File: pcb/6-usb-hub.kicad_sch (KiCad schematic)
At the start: 19 parts, among them J601 USB-C (HRO TYPE-C-31-M-12), U601 CH334P, Y601 12MHz ABM8-272-T3

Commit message: Phase 3: footprint audit fixes and project footprint library
- New project footprint library pcb/scsi-adapter.pretty, generated by
  pcb/_gen/footprints.py from datasheet land patterns: TI RPW0010A (U101/U201),
  Kangnex WJ500V (J101), TE AMPLIMITE .050 HD50 (J302), SHOU HAN TF PUSH
  microSD (J501), Abracon AOTA-B201610 polarized inductor (L401), SHOU HAN
  2-pos DIP (SW301). fp-lib-table added.
- J303 LA header: 2x17 box header C20920, pins 33/34 NC (34-way ribbon to a
  future 2x16 adapter board).
- J302 HD50: TE 5787082-5 squeeze-latch receptacle; shielded symbol, shell to
  GND via R343 0R. TE STEP model git-ignored (pcb/scsi-adapter.3dshapes/).
- D101/D204/D605: D_SMF -> D_SOD-123F (parts are SOD-123FL).
- L401 pins swapped so pad 1 = polarity dot = DVDD_1V1 (RP2350 Fig. 23).
- SW401/SW402: Hroparts K2-1102DP C110153 on SW_PUSH_6mm.
- NOTES, decisions, sources updated; J601 pad question closed; RP2350B
  minimal-design layout copy planned (open question 17).
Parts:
- D605: footprint Diode_SMD:D_SMF -> Diode_SMD:D_SOD-123F
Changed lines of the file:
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@@
 		(property "Reference" "D605" (at 147.32 237.49 270) (effects (font (size 1.27 1.27)) (justify right)))
 		(property "Value" "SMF6.0A" (at 147.32 240.03 270) (effects (font (size 1.27 1.27)) (justify right)))
-		(property "Footprint" "Diode_SMD:D_SMF" (at 144.78 238.76 0) (effects (font (size 1.27 1.27)) (hide yes)))
+		(property "Footprint" "Diode_SMD:D_SOD-123F" (at 144.78 238.76 0) (effects (font (size 1.27 1.27)) (hide yes)))
 		(property "Datasheet" "" (at 144.78 238.76 0) (effects (font (size 1.27 1.27)) (hide yes)))
 		(property "Description" "ESD on VBUS" (at 144.78 238.76 0) (effects (font (size 1.27 1.27)) (hide yes)))

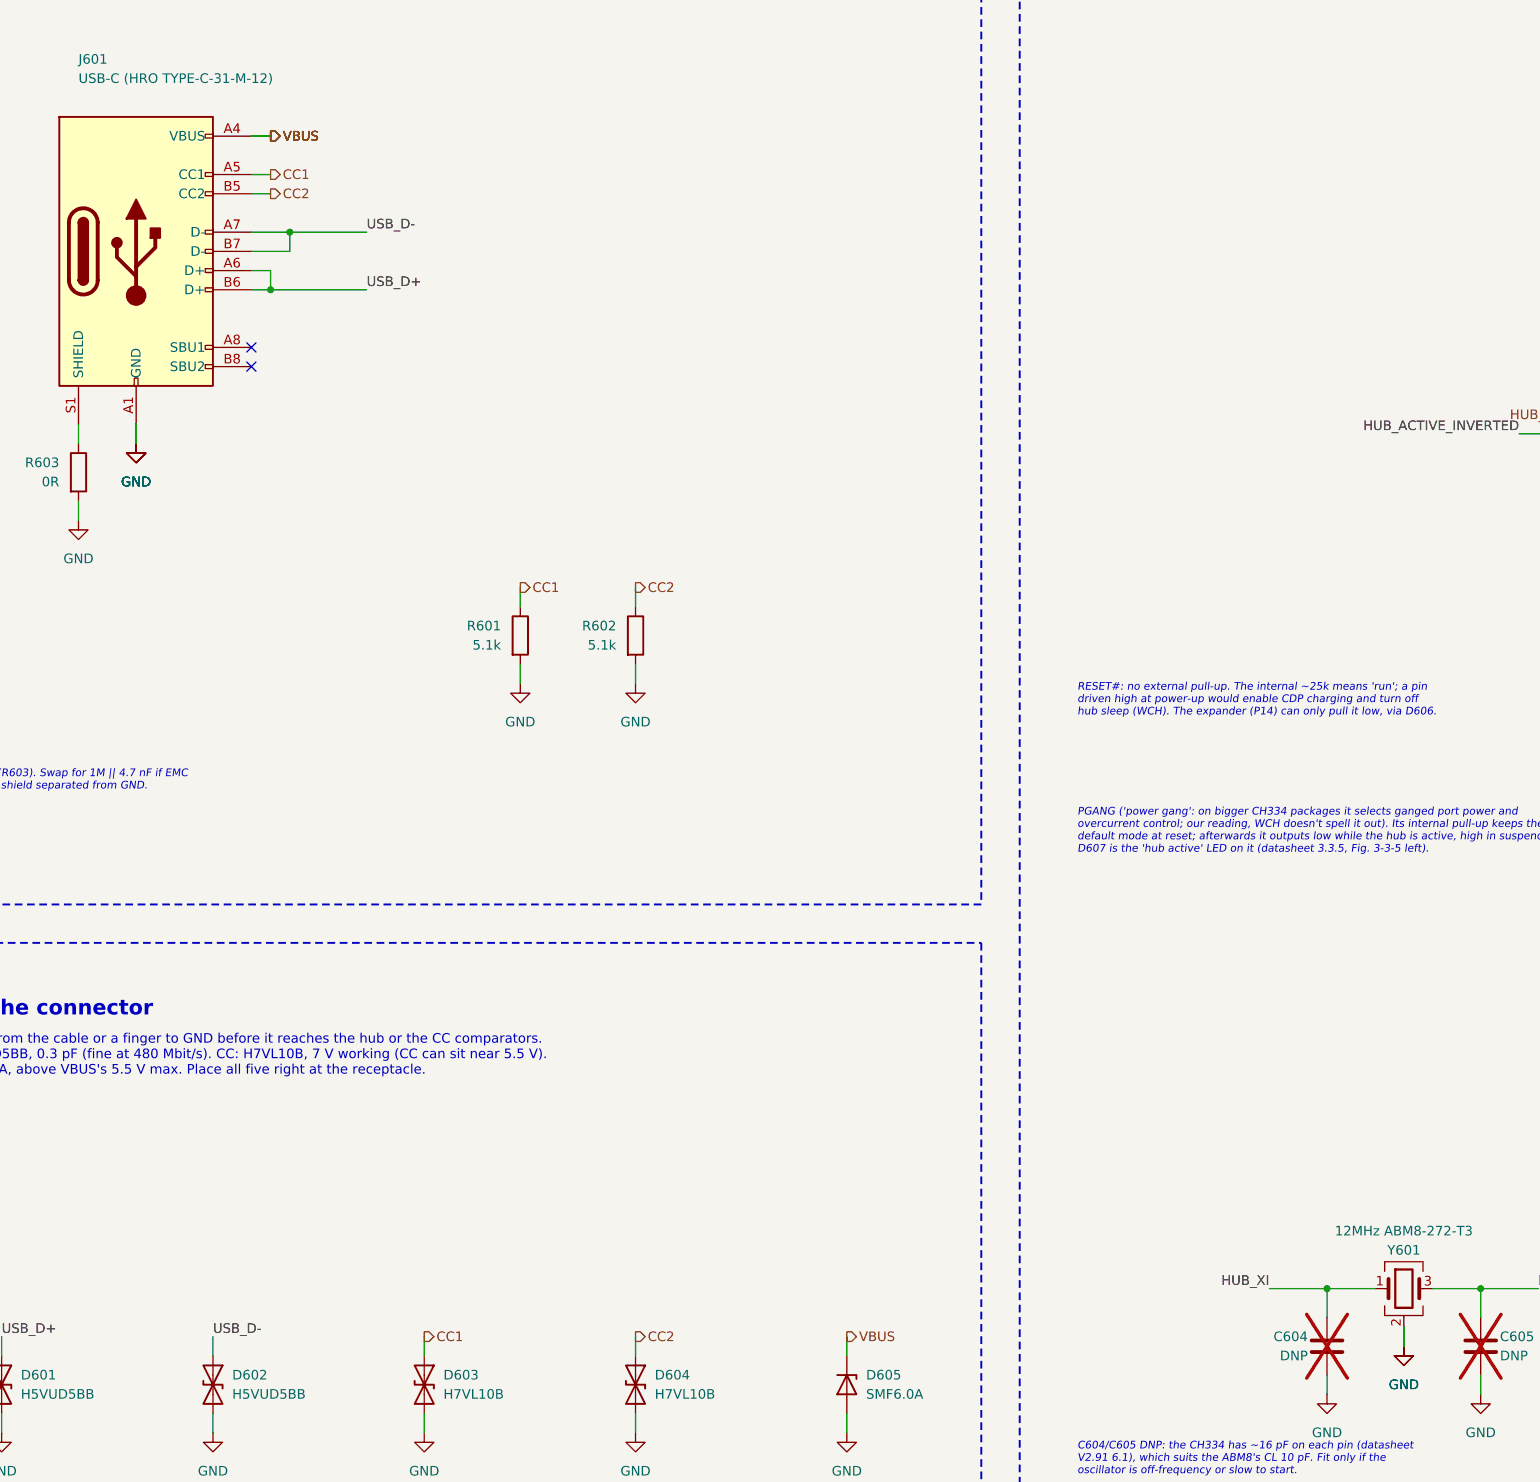
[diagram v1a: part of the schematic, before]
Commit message: route more scsi traces
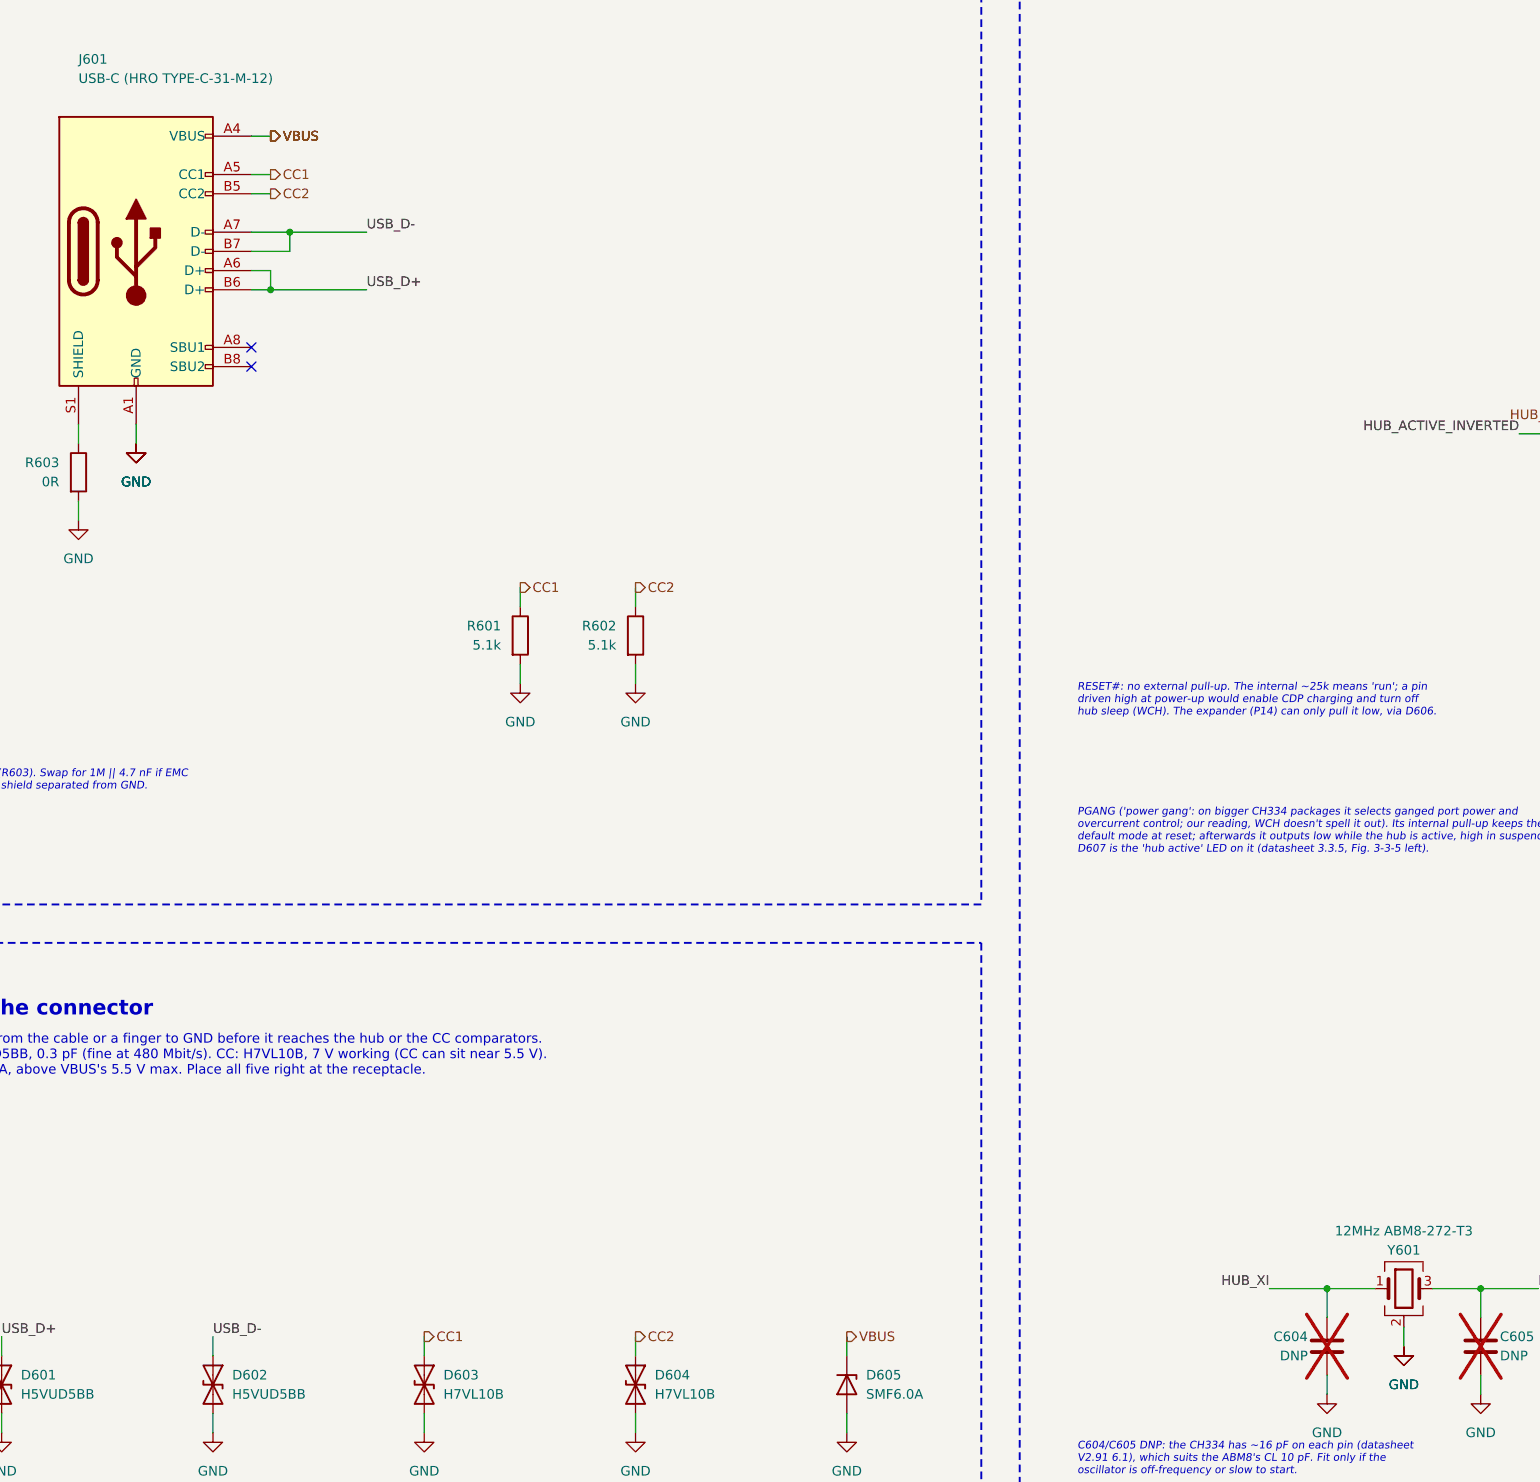
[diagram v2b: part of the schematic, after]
